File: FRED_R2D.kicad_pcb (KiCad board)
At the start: 4 copper layers, 68.4 x 44.9 mm, 87 parts, among them J1 DA15_Receptacle_MountingHoles, J2 RJ45_LED_Shielded, J3 Screw_Terminal_01x07, J4 Conn_01x02_Pin, J5 Conn_01x04, J6 Conn_01x05_Pin, J7 Conn_01x04, Q1 MMBT5551, Q2 MMBT5401, Q3 MMBT5401, Q4 MMBT5551, U1 AD2S1210WDSTZRL7, U2 MC3487DX, U3 AD8662ARZ, U4 74AHC1G86, U5 STM8S003F3P, U6 NCP1117-5.0_SOT223

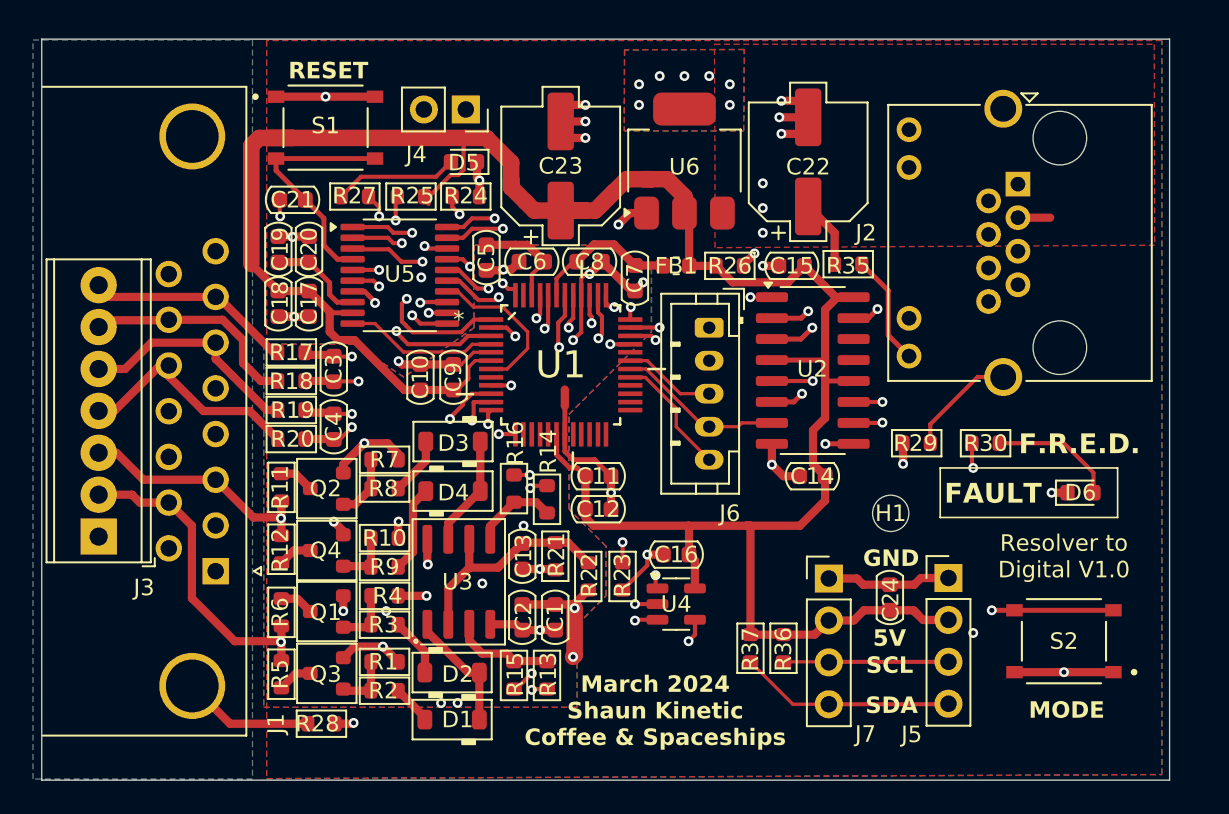
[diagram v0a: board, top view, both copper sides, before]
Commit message: Version 1.1 for mfg
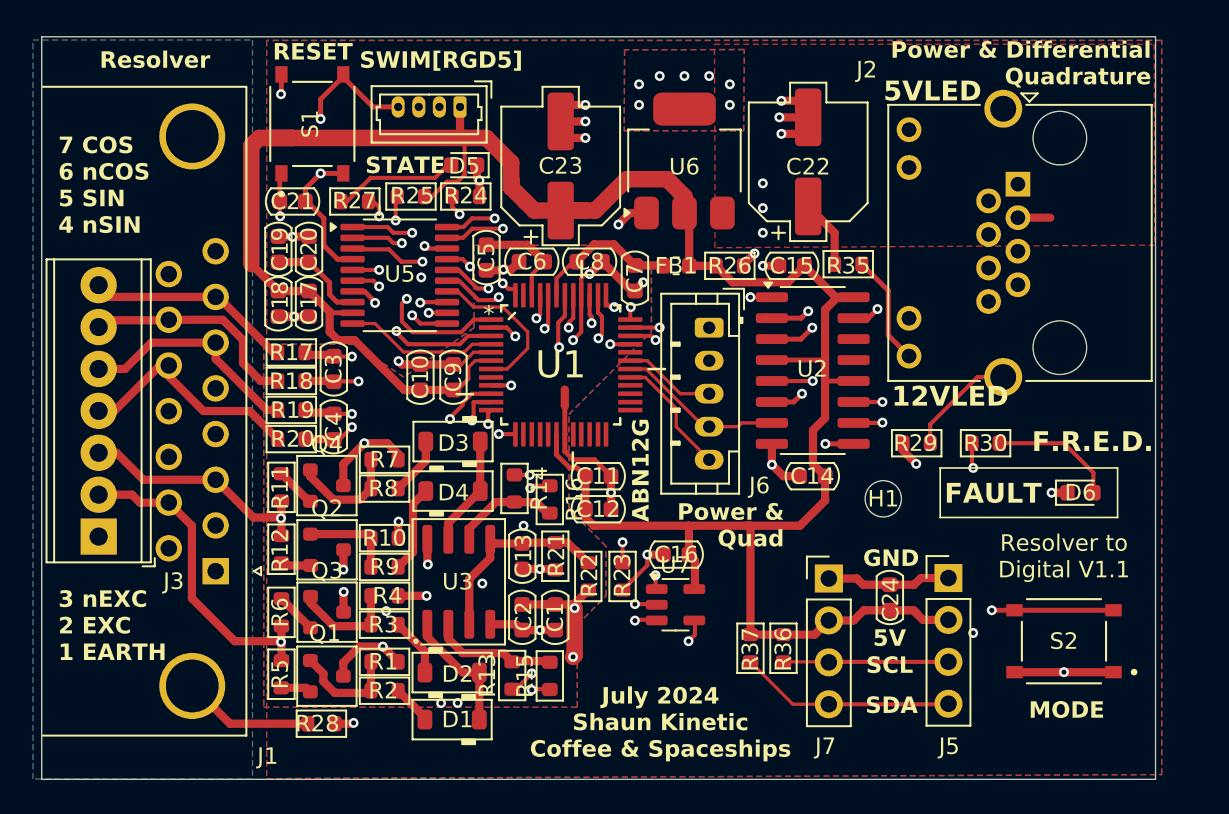
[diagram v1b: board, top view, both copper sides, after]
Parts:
- removed U4: 74AHC1G86, Package_TO_SOT_SMD:SOT-23-5
- added U7: 74AHC1G32, Package_TO_SOT_SMD:SOT-23-5, F.Cu at (147.7, 116.0)
- J4: value Conn_01x02_Pin -> Conn_01x04_Pin; footprint Connector_PinSocket_2.54mm:PinSocket_1x02_P2.54mm_Vertical -> Connector_Molex:Molex_PicoBlade_53047-0410_1x04_P1.25mm_Vertical
- R13, R14: value 15K4 -> 10K
- R15, R16: value 10k -> 15K
- R17, R18, R19, R2, R20, R3, R8, R9: value 3R3 -> 4R7
- R21, R23, R24, R25, R26, R27, R35: value 10k -> 10K
- R22: value 22k -> 22K
- moved Q4 3.93 mm to (126.6, 108.8), turned to 0 degrees
- moved Q1 3.92 mm to (126.6, 120.4), turned to 0 degrees
- moved Q3 3.71 mm to (126.6, 116.5), turned to 0 degrees
- moved Q2 3.71 mm to (126.6, 112.7), turned to 0 degrees
- moved R16 2.27 mm to (140.1, 109.7)
- moved R15 2.17 mm to (140.1, 120.3)
- moved R13 2.11 mm to (137.8, 120.3)
- moved R14 2.08 mm to (137.9, 109.0)
- moved H1 0.99 mm to (160.3, 109.6)
- moved S1 0.83 mm to (125.7, 86.9), turned to 90 degrees
- moved J4 0.38 mm to (134.7, 85.9), turned to 180 degrees
- moved R27 0.30 mm to (128.3, 91.6)
- moved D5 0.20 mm to (134.9, 89.4)
- moved C21 0.10 mm to (124.5, 91.6)
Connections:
- C21 pad 2: Net-(U5-NRST) -> STM_RST
- J4 pad 1: GND -> +5V
- Q1 pad 2: AGND -> Net-(Q1-E)
- Q1 pad 3: Net-(Q1-C) -> +12V
- Q2 pad 2: +12V -> Net-(Q2-E)
- Q2 pad 3: Net-(Q2-C) -> AGND
- Q3 pad 2: +12V -> Net-(Q3-E)
- Q3 pad 3: Net-(Q3-C) -> AGND
- Q4 pad 2: AGND -> Net-(Q4-E)
- Q4 pad 3: Net-(Q4-C) -> +12V
- R1 pad 2: Net-(Q3-B) -> Net-(Q1-B)
- R10 pad 1: Net-(Q4-B) -> Net-(Q2-B)
- R11 pad 1: Net-(Q2-C) -> Net-(Q4-E)
- R12 pad 2: Net-(Q4-C) -> Net-(Q2-E)
- R13 pad 1: EXC_OUT -> EXC
- R13 pad 2: Net-(U3A-+) -> Net-(U3A--)
- R14 pad 1: ~{EXC}_OUT -> ~{EXC}
- R14 pad 2: Net-(U3B-+) -> Net-(U3B--)
- R15 pad 1: EXC -> EXC_OUT
- R15 pad 2: Net-(U3A-+) -> Net-(U3A--)
- R16 pad 1: ~{EXC} -> ~{EXC}_OUT
- R16 pad 2: Net-(U3B-+) -> Net-(U3B--)
- R2 pad 1: Net-(Q3-B) -> Net-(Q1-B)
- R3 pad 2: Net-(Q1-B) -> Net-(Q3-B)
- R4 pad 1: Net-(Q1-B) -> Net-(Q3-B)
- R5 pad 1: Net-(Q3-C) -> Net-(Q1-E)
- R6 pad 2: Net-(Q1-C) -> Net-(Q3-E)
- R7 pad 2: Net-(Q2-B) -> Net-(Q4-B)
- R8 pad 1: Net-(Q2-B) -> Net-(Q4-B)
- R9 pad 2: Net-(Q4-B) -> Net-(Q2-B)
- S1 pad C: Net-(U5-NRST) -> STM_RST
- S1 pad D: Net-(U5-NRST) -> STM_RST
- U3 pad 2: VREF -> Net-(U3A--)
- U3 pad 3: Net-(U3A-+) -> VREF
- U3 pad 5: Net-(U3B-+) -> VREF
- U3 pad 6: VREF -> Net-(U3B--)
- U5 pad 4: Net-(U5-NRST) -> STM_RST
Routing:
- net STM_RST: track 0.00 -> 19.6 mm, vias 0 -> 2
- net Net-(U5-NRST): track 14.6 -> 0.00 mm
- net Net-(U3A--): track 0.00 -> 7.66 mm
- net Net-(U3B--): track 0.00 -> 6.33 mm
- net Net-(U3A-+): track 6.32 -> 0.00 mm
- net Net-(U3B-+): track 5.12 -> 0.00 mm
- net VREF: track 16.7 -> 12.2 mm
- net Net-(Q4-B): track 3.45 -> 6.68 mm
- net Net-(Q3-B): track 3.47 -> 6.64 mm
- net Net-(Q1-B): track 3.49 -> 6.57 mm
- net GND: track 71.3 -> 68.6 mm
- net Net-(Q3-E): track 0.00 -> 2.50 mm
- net Net-(Q4-E): track 0.00 -> 2.45 mm
- net Net-(Q2-C): track 2.12 -> 0.00 mm
- net Net-(Q3-C): track 2.11 -> 0.00 mm
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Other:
- board size 68.4 x 44.9 mm -> 67.5 x 45 mm
- board text added: "12VLED"
- board text added: "3 nEXC 2 EXC 1 EARTH"
- board text added: "5VLED"
- board text added: "7 COS 6 nCOS 5 SIN 4 nSIN"
- board text added: "ABN12G"
- board text added: "July 2024 Shaun Kinetic Coffee & Spaceships"
- board text added: "Power & Differential Quadrature"
- board text added: "Power & Quad"
- board text added: "Resolver"
- board text added: "Resolver to Digital V1.1"
- board text added: "STATE"
- board text added: "SWIM[RGD5]"
- board text removed: "March 2024 Shaun Kinetic Coffee & Spaceships"
- board text removed: "Resolver to Digital V1.0"
